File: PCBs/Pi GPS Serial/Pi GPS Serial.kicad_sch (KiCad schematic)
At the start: 13 parts, among them J1 RS232 OUT, J2 5V In, J3 40HAT, J4 SPI, J5 I2C, J6 Stick Shaker, U1 MAX232

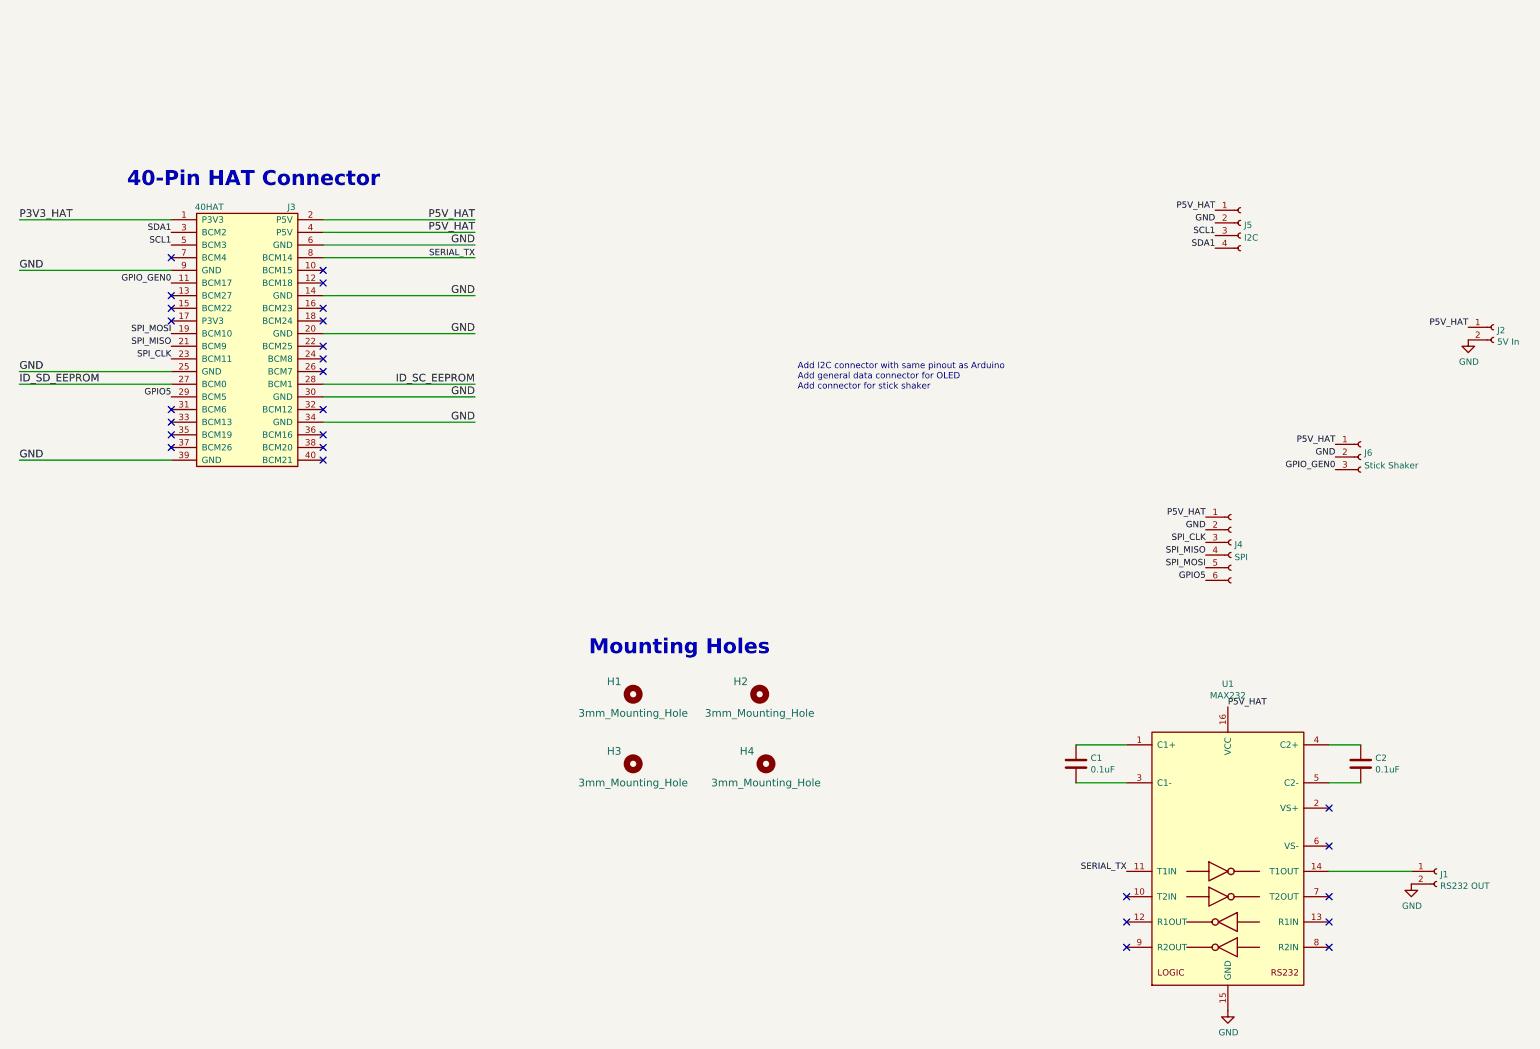
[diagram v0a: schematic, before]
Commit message: Doc
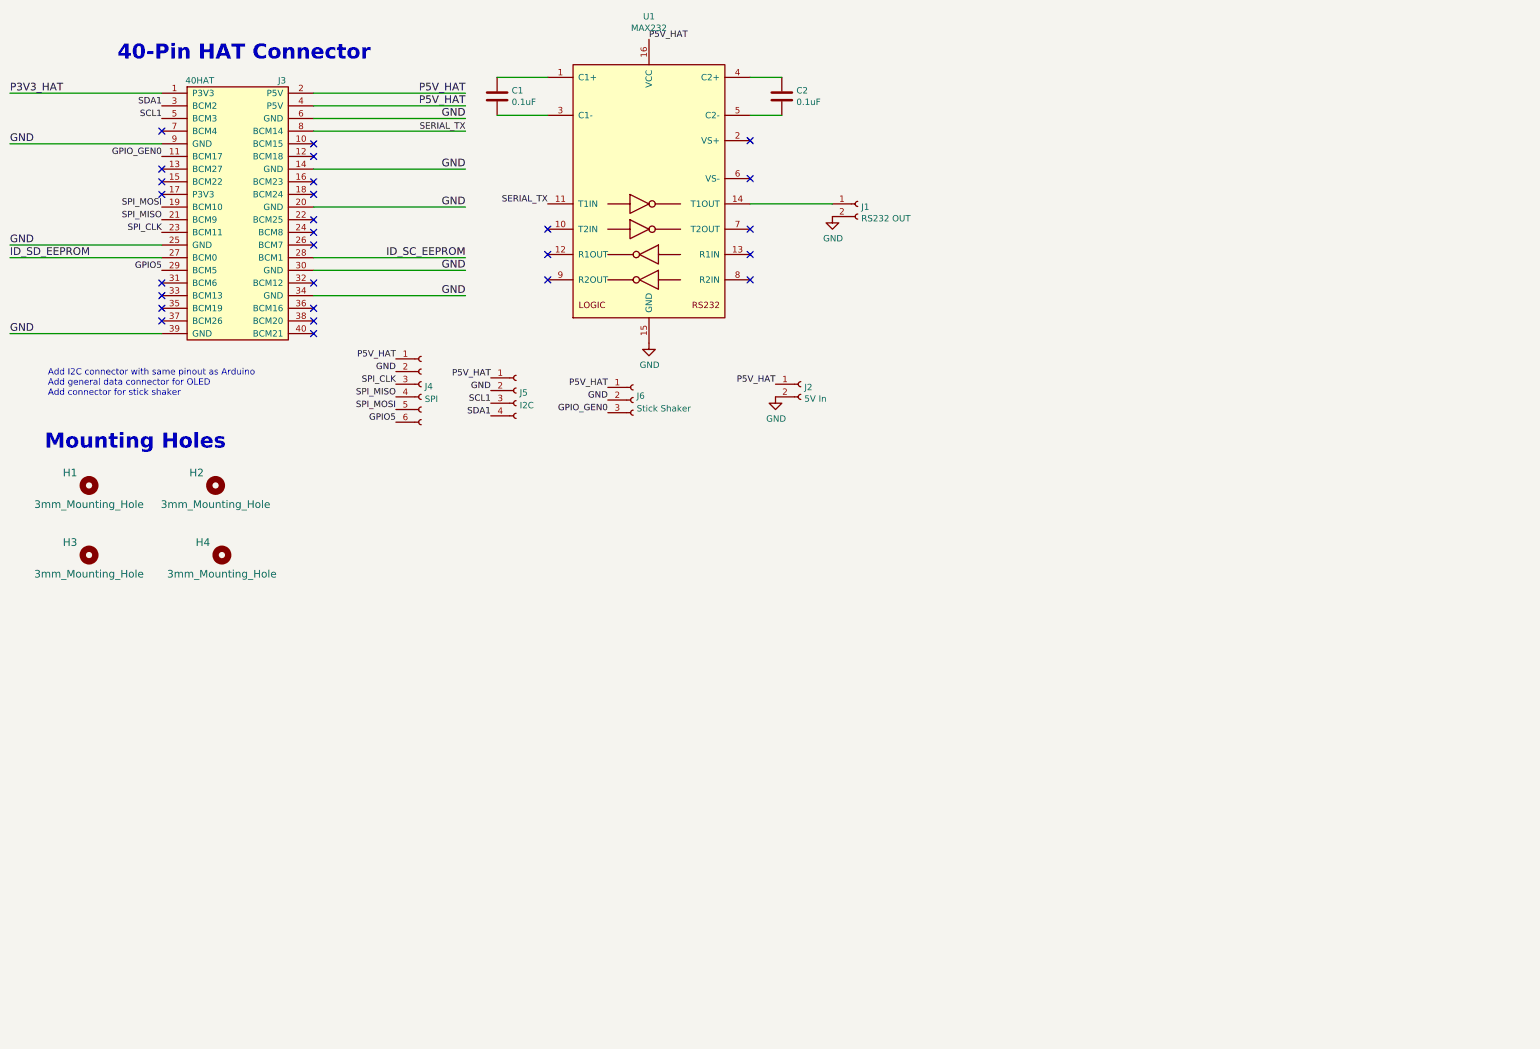
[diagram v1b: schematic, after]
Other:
- moved on the sheet: C1, C2, H1, H2, H3, H4, J1, J2, J3, J4, J5, J6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
